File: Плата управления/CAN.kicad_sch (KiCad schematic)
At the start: 14 parts

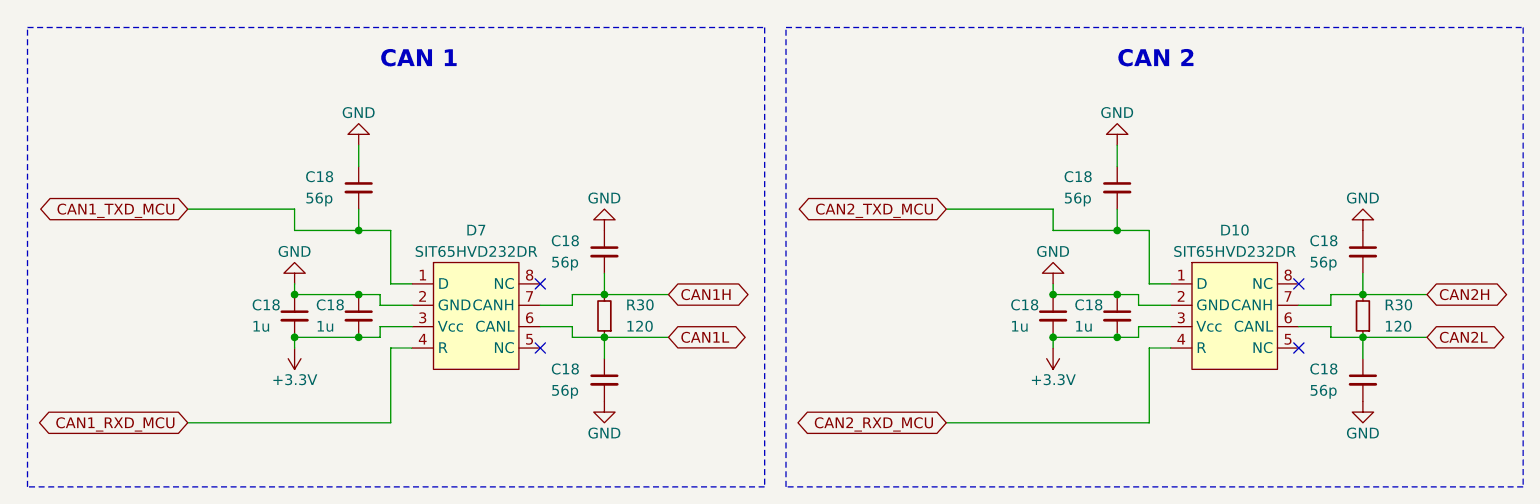
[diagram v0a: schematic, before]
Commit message: Собираю документацию
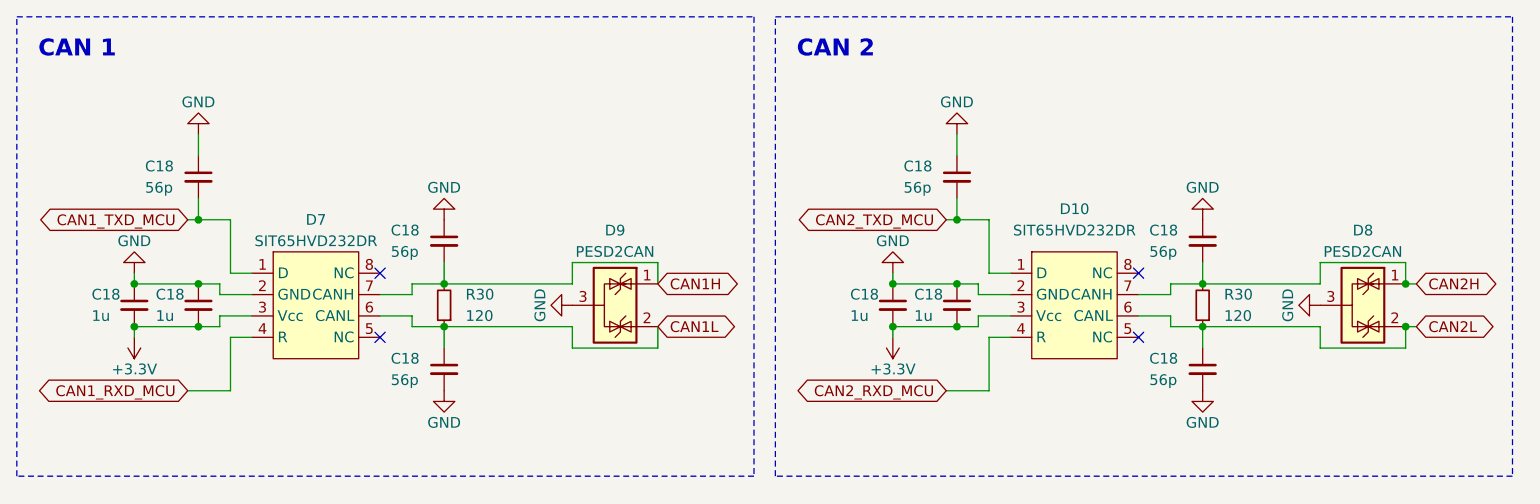
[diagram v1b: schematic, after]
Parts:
- added D8, D9: PESD2CAN, Package_TO_SOT_SMD:SOT-23, symbol Power_Protection:NUP2105L
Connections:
- net CAN1H: now also D9.1 (K)
- net CAN1L: now also D9.2 (K)
- net CAN2H: now also D8.1 (K)
- net CAN2L: now also D8.2 (K)
- net GND: now also D8.3 (A), D9.3 (A)
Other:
- moved on the sheet: C18, D10, D7, R30
